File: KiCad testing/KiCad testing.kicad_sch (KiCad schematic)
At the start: 41 parts, among them J1 USB_A, Q1 IRF540N, Q2 IRF540N, Q3 IRF540N, U1 IR2213, U3 ACS712xLCTR-05B, U4 IR2213

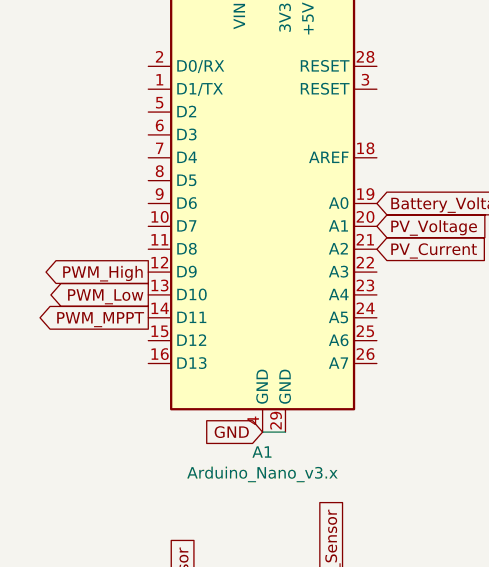
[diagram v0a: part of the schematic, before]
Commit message: Update Schematic
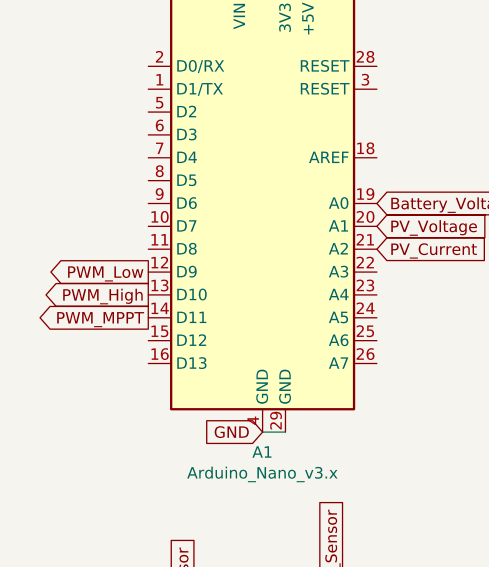
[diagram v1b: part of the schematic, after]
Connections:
- net PWM_High: now also A1.13 (D10); no longer A1.12 (D9)
- net PWM_Low: now also A1.12 (D9); no longer A1.13 (D10)
